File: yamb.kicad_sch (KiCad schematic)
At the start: 14 parts, among them J1 Barrel_Jack, J2 I2C, J3 HEADER, J4 HEADER_2.54, J5 Remote_Reset, J6 Power_Switch, P1 USB_C_Plug_USB2.0, SW1 RESET, U1 TPS3808DBV

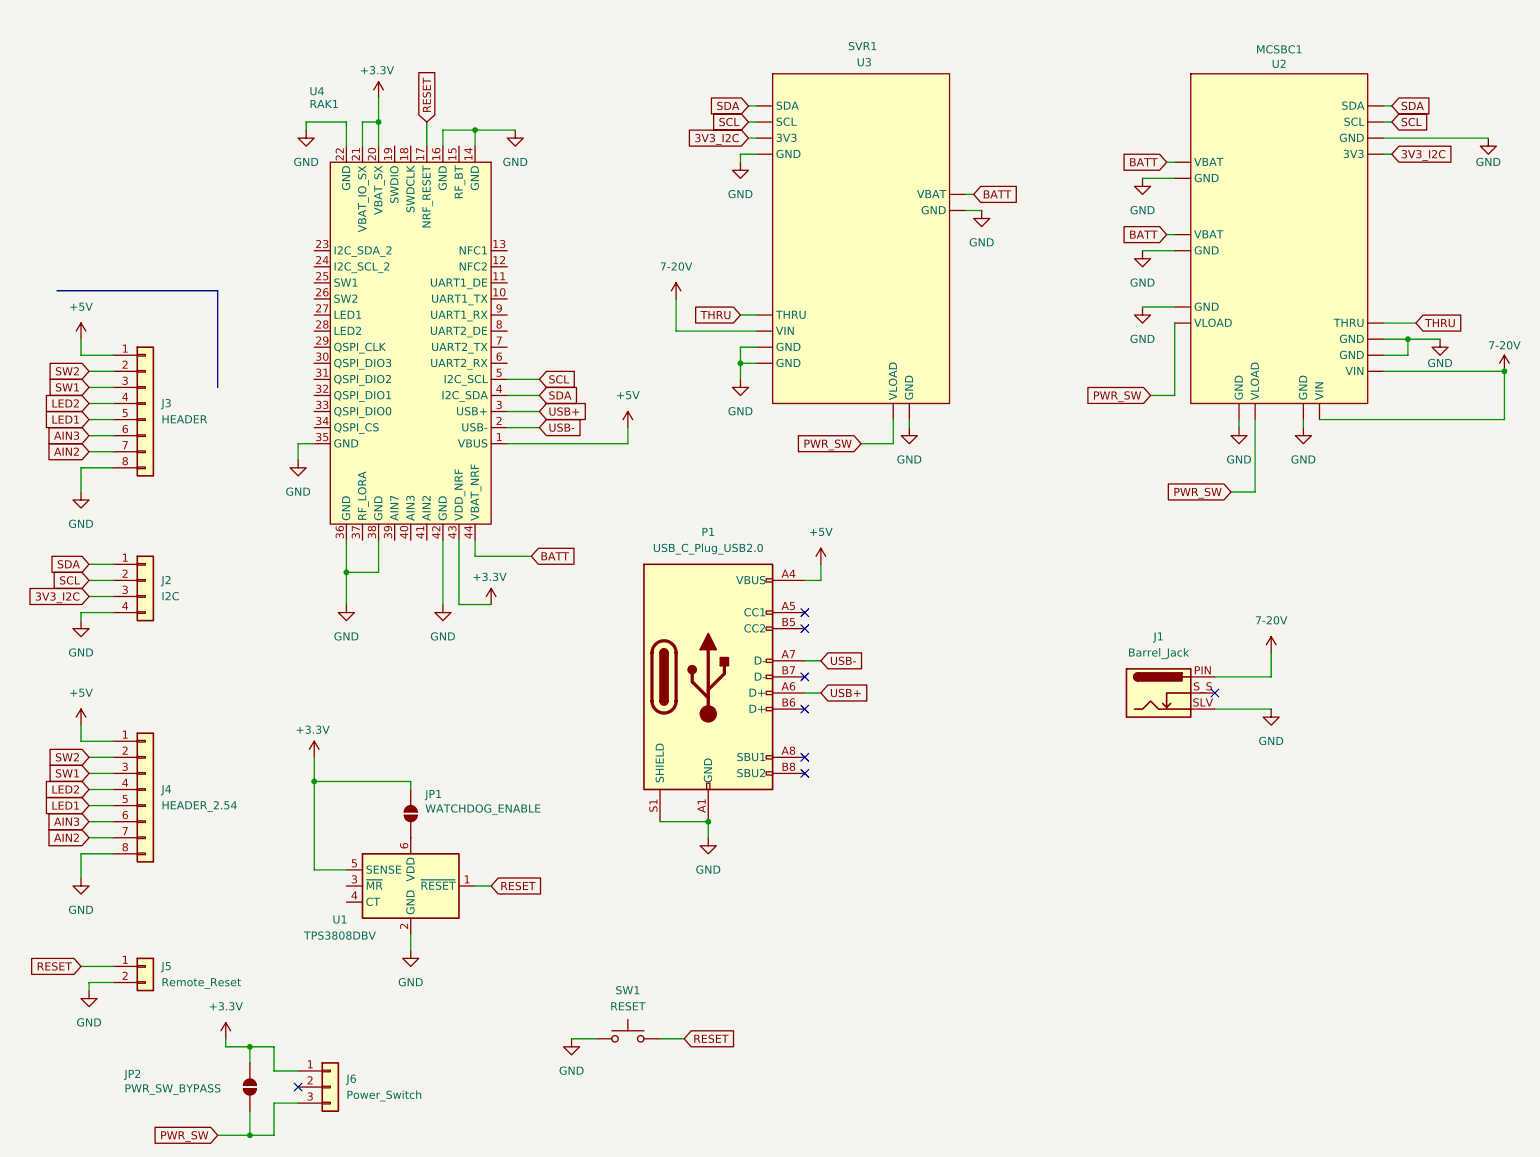
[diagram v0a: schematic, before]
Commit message: custom libraries
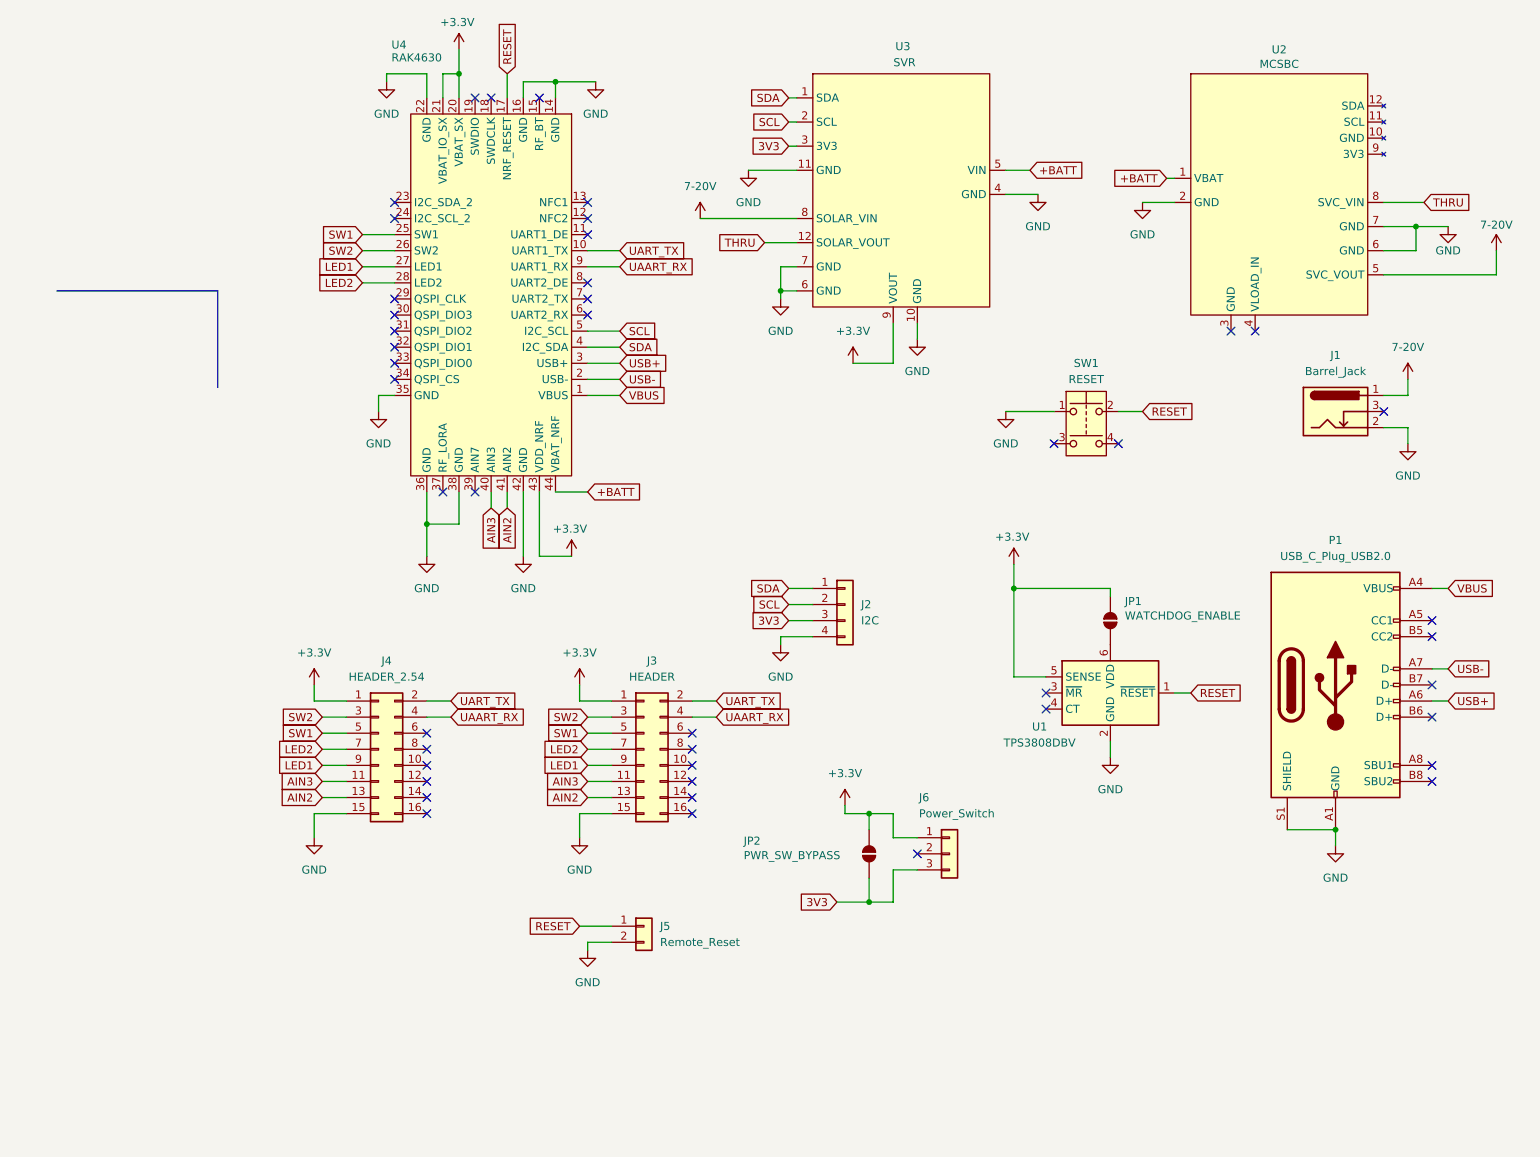
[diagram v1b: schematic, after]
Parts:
- J3: footprint Connector_JST:JST_PH_B8B-PH-K_1x08_P2.00mm_Vertical -> Connector_JST:JST_PHD_B16B-PHDSS_2x08_P2.00mm_Vertical; symbol Connector_Generic:Conn_01x08 -> Connector_Generic:Conn_02x08_Odd_Even
- J4: footprint Connector_PinHeader_2.54mm:PinHeader_1x08_P2.54mm_Vertical -> Connector_PinHeader_2.54mm:PinHeader_2x08_P2.54mm_Vertical; symbol Connector_Generic:Conn_01x08 -> Connector_Generic:Conn_02x08_Odd_Even
- SW1: symbol Switch:SW_Push -> Switch:SW_Push_Dual
- U2: renamed from MCSBC1; value U2 -> MCSBC; symbol Regulator_Controller:VOLTAIC_SOLAR_1 -> Andy_Symbols:VOLTAIC_MCSBC
- U3: renamed from SVR1; value U3 -> SVR; footprint Converter_DCDC:Voltaic_SVR -> Andy_Footprints:Voltaic_SVR; symbol Regulator_Controller:VOLTAIC_SVR -> Andy_Symbols:VOLTAIC_SVR
- U4: renamed from RAK1; value U4 -> RAK4630; footprint RF_Module:RAK4630 -> Andy_Footprints:RAK4630; symbol RF_Module:RAK4630 -> Andy_Symbols:RAK4630
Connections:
- net +3.3V: now also J3.1 (Pin_1), J4.1 (Pin_1), U3.9 (VOUT)
- net 7-20V: now also J1.1, U2.5 (SVC_VOUT); no longer J1.PIN, U2.13 (VIN), U2.18 (VIN)
- net AIN2: now also J3.13 (Pin_13), J4.13 (Pin_13), U4.41 (AIN2); no longer J3.7 (Pin_7), J4.7 (Pin_7)
- net AIN3: now also J3.11 (Pin_11), J4.11 (Pin_11), U4.40 (AIN3); no longer J3.6 (Pin_6), J4.6 (Pin_6)
- net GND: now also J1.2, J3.15 (Pin_15), J4.15 (Pin_15), U2.2 (GND), U2.7 (GND); no longer J1.SLV, J3.8 (Pin_8), J4.8 (Pin_8), U2.10 (GND), U2.12 (GND), U2.14 (GND), U2.16 (GND), U2.17 (GND), U2.4 (GND), U2.8 (GND)
- net LED1: now also J3.9 (Pin_9), J4.9 (Pin_9), U4.27 (LED1); no longer J3.5 (Pin_5), J4.5 (Pin_5)
- net LED2: now also J3.7 (Pin_7), J4.7 (Pin_7), U4.28 (LED2); no longer J3.4 (Pin_4), J4.4 (Pin_4)
- net SCL: no longer U2.2 (SCL)
- net SDA: no longer U2.1 (SDA)
- net SW1: now also J3.5 (Pin_5), J4.5 (Pin_5), U4.25 (SW1); no longer J3.3 (Pin_3), J4.3 (Pin_3)
- net SW2: now also J3.3 (Pin_3), J4.3 (Pin_3), U4.26 (SW2); no longer J3.2 (Pin_2), J4.2 (Pin_2)
- net THRU: now also U2.8 (SVC_VIN); no longer U2.15 (THRU)
- net UART_TX: now reaches U4.10 (UART1_TX)
- net UART_TX: now also J3.2 (Pin_2), J4.2 (Pin_2)
- net UAART_RX: now reaches U4.9 (UART1_RX)
- net UAART_RX: now also J3.4 (Pin_4), J4.4 (Pin_4)
- net +5V renamed VBUS
- net VBUS: no longer J3.1 (Pin_1), J4.1 (Pin_1)
- net 3V3_I2C renamed 3V3
- net 3V3: now also J6.3 (Pin_3), JP2.2 (B); no longer U2.3 (3V3)
- net BATT renamed +BATT
- net +BATT: now also U2.1 (VBAT); no longer U2.5 (VBAT), U2.7 (VBAT)
- removed net PWR_SW: J6.3 (Pin_3), JP2.2 (B), U2.11 (VLOAD), U2.9 (VLOAD), U3.9 (VLOAD)
- no-connect marks 8 -> 45
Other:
- moved on the sheet: J1, J2, J5, J6, JP1, JP2, P1, U1, U4
